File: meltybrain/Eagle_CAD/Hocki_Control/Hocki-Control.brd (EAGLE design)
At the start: 87 x 44 mm, 105 parts, among them J1 SM05B-SRSS-TB(LF)(SN), J2 SM05B-SRSS-TB(LF)(SN), U1 TEENSY_4.1, U10 TLV3502AIDCNR, U11 NL27WZ32USG, U12 NL27WZ32USG, U13 HMC1052L-TR, U14 LMV358, U15 IRF7509, U16 TMUX1219DCKR, U17 LMV358, U18 LMV358, U19 AP2210K-3.3TRG1, U2 ADXL375, U20 AP2210K-5.0TRG1, U3 ADXL375, U4 ADXL375, U5 ADXL375, U6 LMH6612MAX/NOPB, U7 LMH6612MAX/NOPB, U8 LMH6612MAX/NOPB, U9 LMH6612MAX/NOPB

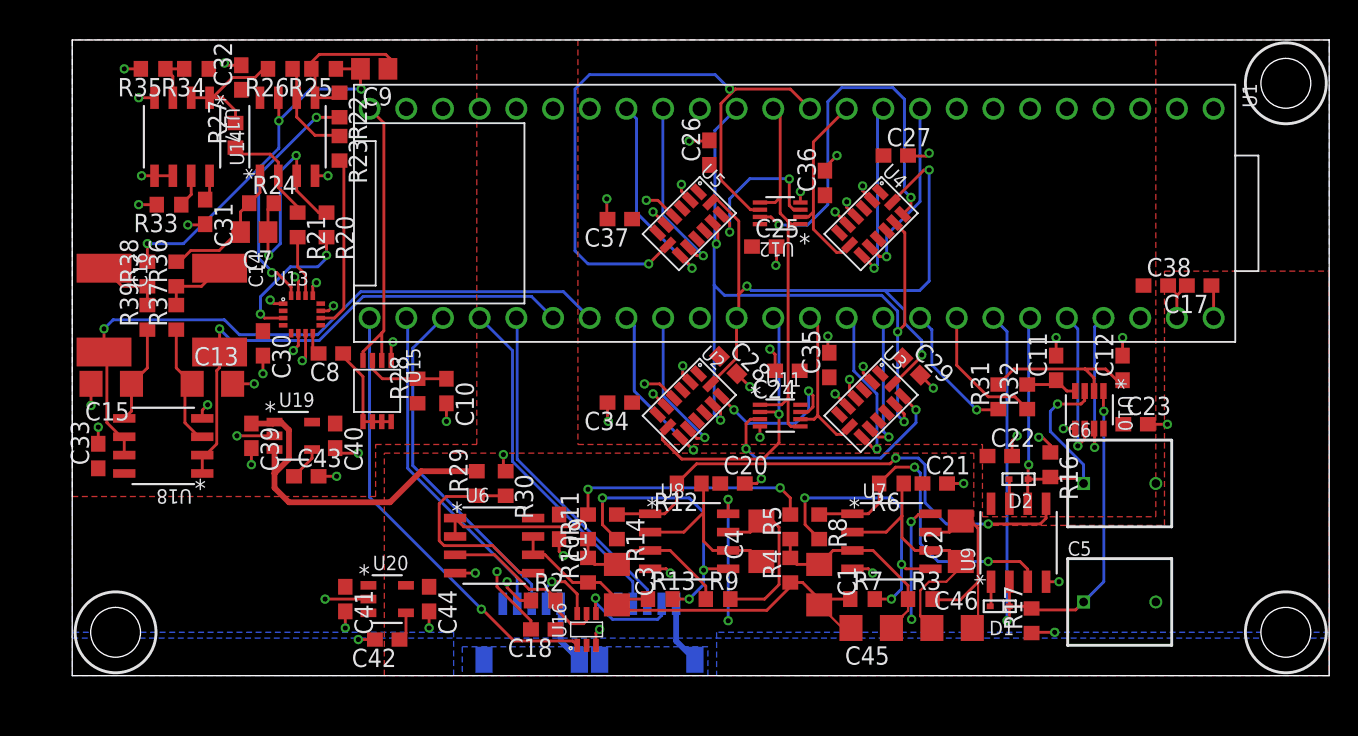
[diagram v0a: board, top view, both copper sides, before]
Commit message: forgot to save before pushing...
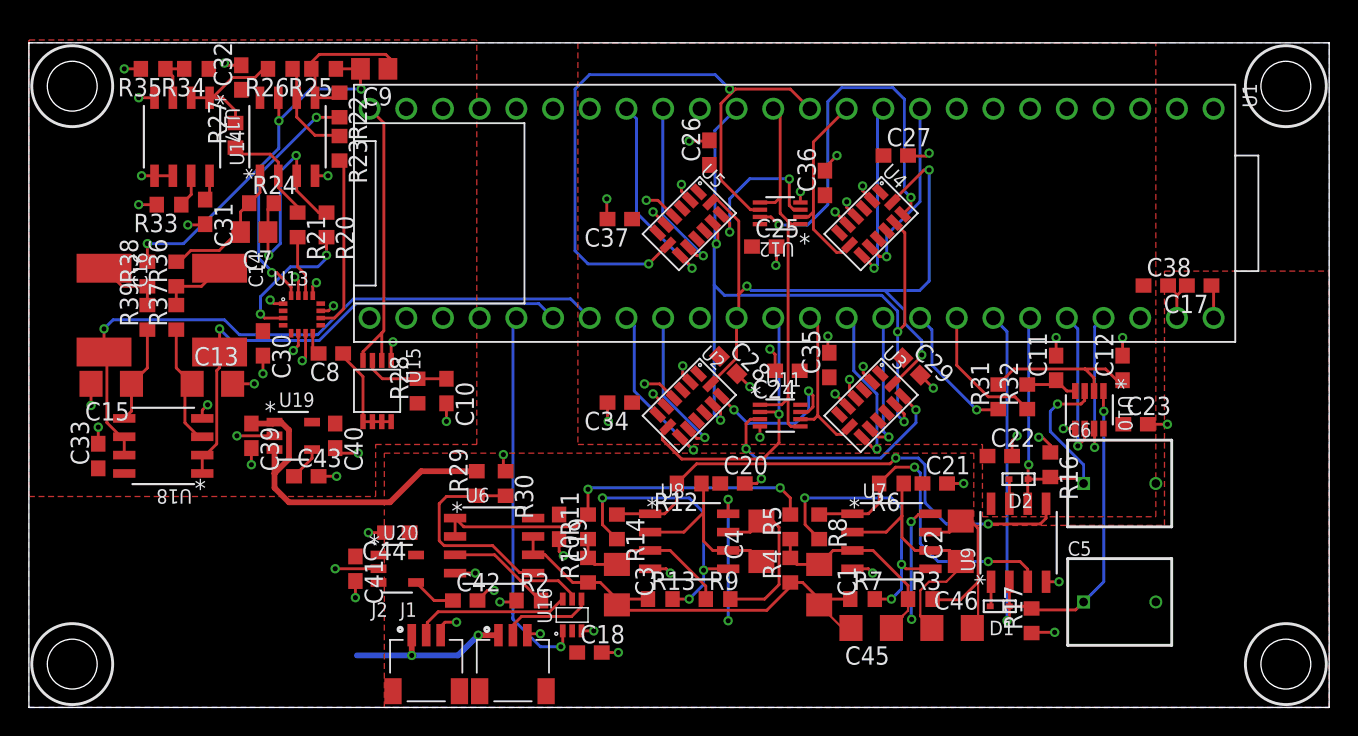
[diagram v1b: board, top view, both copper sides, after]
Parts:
- J1, J2: value SM05B-SRSS-TB(LF)(SN) -> SM03B-SRSS-TB(LF)(SN); device Hocki_Library:SM05B-SRSS-TB(LF)(SN) -> Hocki_Library:SM03B-SRSS-TB(LF)(SN)
- moved J1 9.45 mm to (-18.5, -22.2), flipped to the top
- moved J2 7.50 mm to (-24.5, -22.2), flipped to the top
- moved C42 6.04 mm to (-21.8, -19.8), turned to 0 degrees
- moved C44 5.10 mm to (-26.5, -15.1), turned to 180 degrees
- moved C18 3.58 mm to (-13.2, -23.4), turned to 0 degrees
- moved C41 2.21 mm to (-29.4, -17.6)
- moved U20 2.21 mm to (-26.5, -17.6)
- moved U16 1.41 mm to (-14.4, -20.8)
- moved R2 1.00 mm to (-17.4, -19.8)
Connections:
- removed net IR_BOTTOM_A0: J2.3, U1.35
- removed net IR_BOTTOM_A1: J2.4, U1.34
- removed net IR_TOP_A0: J1.3, U1.37
- removed net IR_TOP_A1: J1.4, U1.36
- net 5V: now also J1.S1, J1.S2, J2.S1, J2.S2
- net 9V: no longer J1.S1, J1.S2, J2.S1, J2.S2
- net GND: now also J1.3, J2.3; no longer J1.5, J2.5
- net IR_SEL: now also U1.37; no longer U1.33
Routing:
- net IR_TOP_A1: track 24.2 -> 0.00 mm
- net IR_BOTTOM_A0: track 24.1 -> 0.00 mm
- net IR_TOP_A0: track 23.6 -> 0.00 mm
- net IR_BOTTOM_A1: track 23.0 -> 0.00 mm
- net IR_BOTTOM: track 5.14 -> 10.8 mm, vias 1 -> 0
- net IR_SEL: track 31.0 -> 26.2 mm
- net 9V: track 8.87 -> 11.8 mm, vias 0 -> 2
- net GND: track 105.4 -> 103.1 mm, vias 70 -> 72
- net N$8: track 2.04 -> 3.07 mm
- net IR_TOP: track 7.36 -> 6.50 mm, vias 1 -> 0
- net VG_SIGNAL: track 12.1 -> 11.5 mm
- removed copper zone on layer 16, net 9V
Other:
- board size 87 x 44 mm -> 90 x 46 mm
